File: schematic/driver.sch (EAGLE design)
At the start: 137 parts, among them IC1 DW01A, IC2 DW01A, IC3 DW01A, IC4 MPU6050, Q2 SI1922EDH-T1-GE3, Q3 SI1922EDH-T1-GE3, Q4 SI1922EDH-T1-GE3

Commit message: Pull up resistors to two I2C buses
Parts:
- added R47: 4.7k, rcl:R-EU_R0805
- added R48: 4.7, rcl:R-EU_R0805
- R15: value 4k7 -> 4.7k
- R16: value 4k7 -> 4.7
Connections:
- net SCL: no longer IC4G$1.SCL, R16.1
- net SCL1: now also IC4G$1.SCL, R47.1
- net SCL2: now also R15.1
- net SDA: no longer IC4G$1.SDA, R15.1
- net SDA1: now also IC4G$1.SDA, R48.1
- net SDA2: now also R16.1
- net VCC: no longer R15.2, R16.2
- net VDD: now also R15.2, R16.2, R47.2, R48.2
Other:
- moved on the sheet: C22, C23, C24, C25, C26, IC4, JP10, JP3, JP5, JP6, JP7, JP8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

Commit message: ułożenie pinów i podpięcie sterowników rage quit
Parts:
- removed 3.3V1, 3.3V2, 3.3V3: (no value), led:LEDCHIPLED_0805
- removed C15: 100n, rcl:C-EUC0603
- removed I2C_CON: (no value), pinhead:PINHD-1X4
- removed R5, R6, R9: 1k, rcl:R-EU_R0805
- added BATTERY: (no value), pinhead:PINHD-1X2
- added CELLS: S4B-XH-A(LF)(SN), Connectors:S4B-XH-A(LF)(SN)
- added JP11, JP12: (no value), pinhead:PINHD-1X3
- added JP13, JP14: (no value), pinhead:PINHD-1X4
- added _C7: 100n, rcl:C-EUC0603
- added _C9: 1uF, rcl:C-EUC0603
- D2, D3, D4, D5, D6, D7: value S3A -> (none); device s3x_10:S3A -> adafruit:LEDCHIPLED-0603-TTW
- JP2: device pinhead:PINHD-1X2 -> pinhead:PINHD-2X14
- Q2: value SI1922EDH-T1-GE3 -> MOSFET1
- Q3: value SI1922EDH-T1-GE3 -> MOSFET2
- Q4: value SI1922EDH-T1-GE3 -> MOSFET3
- _C8: value 100n -> 10n
- renumbered C1 to _C3, C10 to _C1, C11 to _C2, C16 to _C6, C2 to _C8, C4 to _C4, C5 to _C5, JP10 to DIS7, JP3 to DIS1, JP5 to DIS2, JP6 to DIS3, JP7 to DIS4, JP8 to DIS5, JP9 to DIS6, Q1 to XTAL
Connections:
- removed net AO1: MB.1, U$7.A02, U$7.A02., U$7.B02, U$7.B02.
- removed net N$48: C27.1, C28.1, U$6.VM1
- removed net N$52: 3.3V2.C, R6.2
- removed net N$53: 3.3V3.C, R5.2
- removed net N$57: STM32PORTB_L.PB5
- removed net SCL: I2C_CON.2
- removed net SDA: I2C_CON.1
- removed net VSS: STM32AN_POWER.VSSA
- new net ...: STM32PORTB_H.PB12
- new net ADC5: JP11.3, STM32PORTB_L.PB3
- new net ADC6: JP12.3, STM32PORTB_L.PB4
- new net N$17: JP14.3
- new net N$64: MB.2, U$7.A02, U$7.A02., U$7.B02, U$7.B02.
- net A01: now also MA.1; no longer MA.2
- net A02: now also MB.1; no longer MB.2
- net ADC4: now also STM32PORTB_L.PB1
- net AO2: now also MA.2; no longer MA.1
- net BAT+: now also BATTERY.2; no longer JP2.2
- net BAT_ON: now also C27.1, C28.1, U$6.VM1
- net BUT: no longer STM32PORTB_L.PB0
- net CELL1: now also CELLS.2
- net CELL2: now also CELLS.3
- net CELL3: now also CELLS.4
- net GND: now also BATTERY.1, CELLS.1, JP11.2, JP12.2, JP13.3, S2.1, S2.2, S2.3, STM32AN_POWER.VSSA, _C7.2, _C9.2; no longer C15.2, I2C_CON.3, JP2.1, R5.1, R6.1, R9.1
- net INT: now also STM32PORTB_L.PB0; no longer STM32PORTB_L.PB1
- net LED1: no longer STM32PORTB_L.PB3, STM32PORTB_L.PB4
- net MA1: now also STM32PORTB_L.PB5; no longer STM32PORTB_H.PB12
- net MA2: now also STM32PORTB_H.PB8; no longer STM32PORTB_H.PB9
- net N$2: now also JP14.4; no longer 3.3V1.C, R9.2
- net PWMA: now also STM32PORTB_H.PB9; no longer STM32PORTB_H.PB8
- net SCL2: now also JP13.2
- net SDA2: now also JP13.1
- net SW1: no longer 3.3V3.A, S2.1
- net SW2: no longer 3.3V2.A, S2.2
- net SW3: no longer 3.3V1.A, S2.3
- net SWDA: now also STM32PORTA_H.PA13
- net SWDIO: no longer STM32PORTA_H.PA13
- net VCC: now also JP11.1, JP12.1, JP13.4
- net VCC_S: no longer I2C_CON.4
- net VDD: now also _C7.1, _C9.1; no longer C15.1
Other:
- note added: "Czujniki"

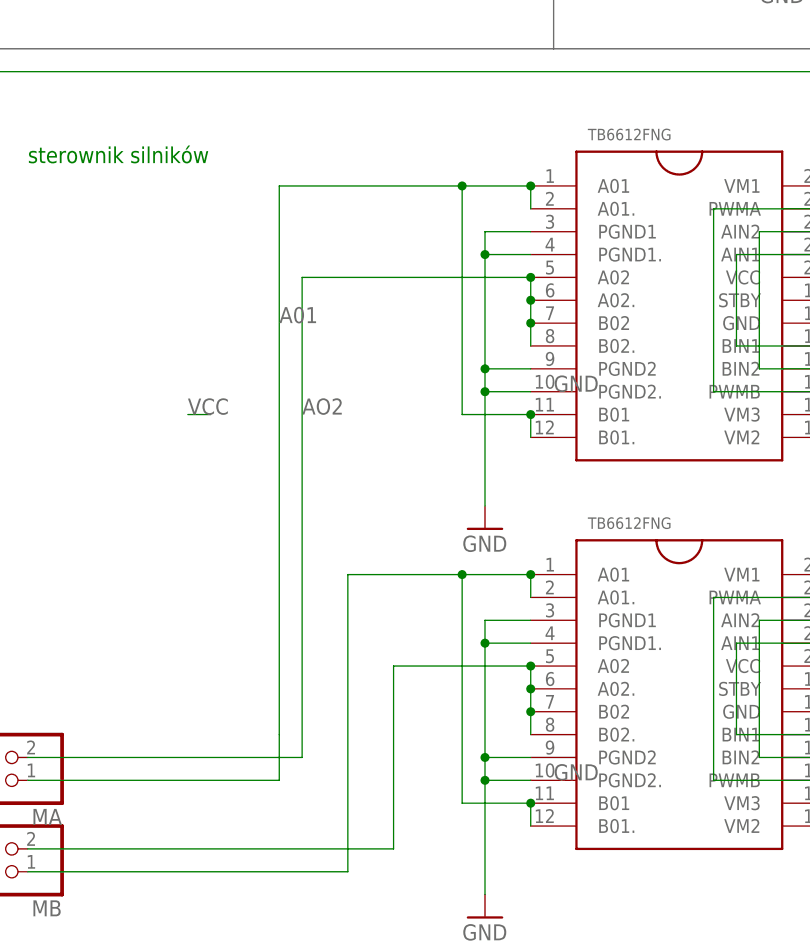
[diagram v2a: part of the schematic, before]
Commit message: s
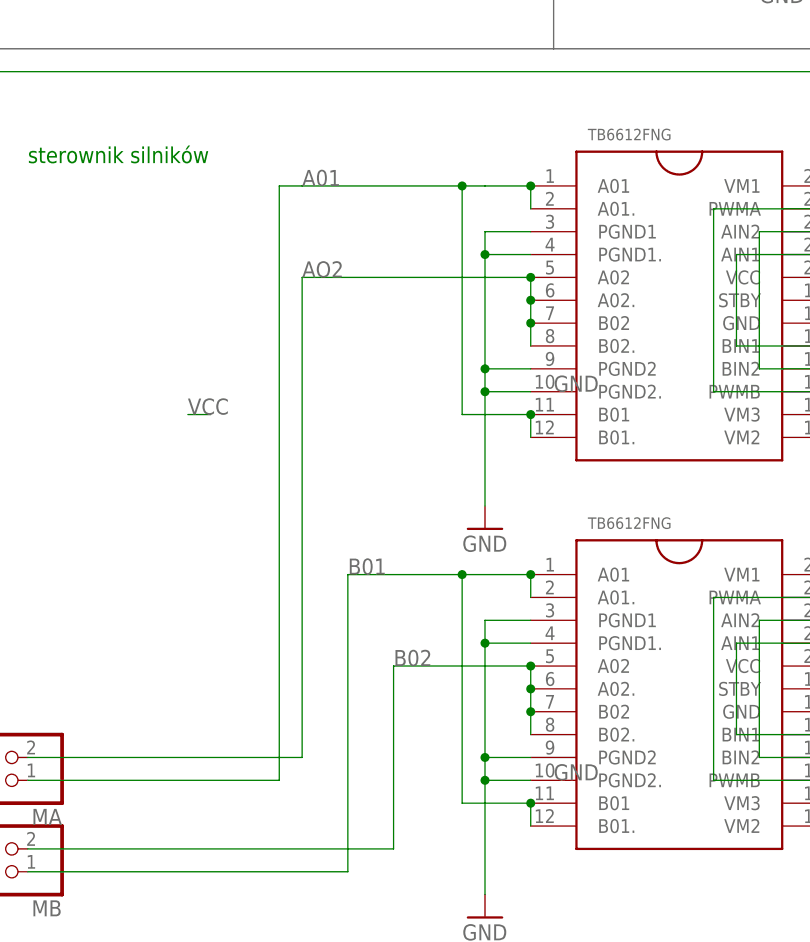
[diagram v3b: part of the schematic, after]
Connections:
- net A02 renamed B01
- net N$64 renamed B02
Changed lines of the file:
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@@
 <junction x="-7.62" y="38.1"/>
 <wire x1="-7.62" y1="35.56" x2="-7.62" y2="38.1" width="0.1524" layer="91"/>
-<label x="-33.02" y="27.94" size="1.778" layer="95"/>
+<label x="-33.02" y="43.18" size="1.778" layer="95"/>
 <junction x="-7.62" y="43.18"/>
 <wire x1="-7.62" y1="43.18" x2="-33.02" y2="43.18" width="0.1524" layer="91"/>
@@
 <wire x1="-7.62" y1="25.4" x2="-7.62" y2="27.94" width="0.1524" layer="91"/>
 <junction x="-7.62" y="27.94"/>
-<label x="-35.56" y="38.1" size="1.778" layer="95"/>
+<label x="-33.02" y="53.34" size="1.778" layer="95"/>
 <wire x1="-7.62" y1="53.34" x2="-7.62" y2="50.8" width="0.1524" layer="91"/>
-<wire x1="-7.62" y1="53.34" x2="-15.24" y2="53.34" width="0.1524" layer="91"/>
+<wire x1="-7.62" y1="53.34" x2="-12.7" y2="53.34" width="0.1524" layer="91"/>
 <junction x="-7.62" y="53.34"/>
-<wire x1="-35.56" y1="53.34" x2="-35.56" y2="-7.62" width="0.1524" layer="91"/>
+<wire x1="-35.56" y1="53.34" x2="-35.56" y2="-12.7" width="0.1524" layer="91"/>
 <junction x="-15.24" y="53.34"/>
-<wire x1="-35.56" y1="-7.62" x2="-35.56" y2="-10.16" width="0.1524" layer="91"/>
-<wire x1="-15.24" y1="53.34" x2="-35.56" y2="53.34" width="0.1524" layer="91"/>
+<wire x1="-15.24" y1="53.34" x2="-33.02" y2="53.34" width="0.1524" layer="91"/>
 <pinref part="U$6" gate="G$1" pin="A01"/>
 <pinref part="U$6" gate="G$1" pin="A01."/>
@@
 <pinref part="U$6" gate="G$1" pin="B01."/>
 <pinref part="MA" gate="G$1" pin="1"/>
-<wire x1="-35.56" y1="-10.16" x2="-35.56" y2="-12.7" width="0.1524" layer="91"/>
+<wire x1="-33.02" y1="53.34" x2="-35.56" y2="53.34" width="0.1524" layer="91"/>
 <wire x1="-35.56" y1="-12.7" x2="-63.5" y2="-12.7" width="0.1524" layer="91"/>
-</segment>
-</net>
-<net name="A02" class="0">
+<wire x1="-12.7" y1="53.34" x2="-15.24" y2="53.34" width="0.1524" layer="91"/>
+</segment>
+</net>
+<net name="B01" class="0">
 <segment>
 <wire x1="-15.24" y1="10.16" x2="-15.24" y2="-15.24" width="0.1524" layer="91"/>
@@
 <pinref part="MB" gate="G$1" pin="1"/>
 <wire x1="-27.94" y1="-22.86" x2="-63.5" y2="-22.86" width="0.1524" layer="91"/>
+<label x="-27.94" y="10.16" size="1.778" layer="95"/>
 </segment>
 </net>
@@
 </segment>
 </net>
-<net name="N$64" class="0">
+<net name="B02" class="0">
 <segment>
 <junction x="-7.62" y="-2.54"/>
@@
 <wire x1="-22.86" y1="0" x2="-22.86" y2="-20.32" width="0.1524" layer="91"/>
 <wire x1="-22.86" y1="-20.32" x2="-63.5" y2="-20.32" width="0.1524" layer="91"/>
-</segment>
-</net>
+<label x="-22.86" y="0" size="1.778" layer="95"/>
+</segment>
+</net>
